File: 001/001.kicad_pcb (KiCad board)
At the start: 2 copper layers, 47.6 x 49.1 mm, 8 parts, among them U1 MF-Jalisco, U2 Firma, U3 PinBase

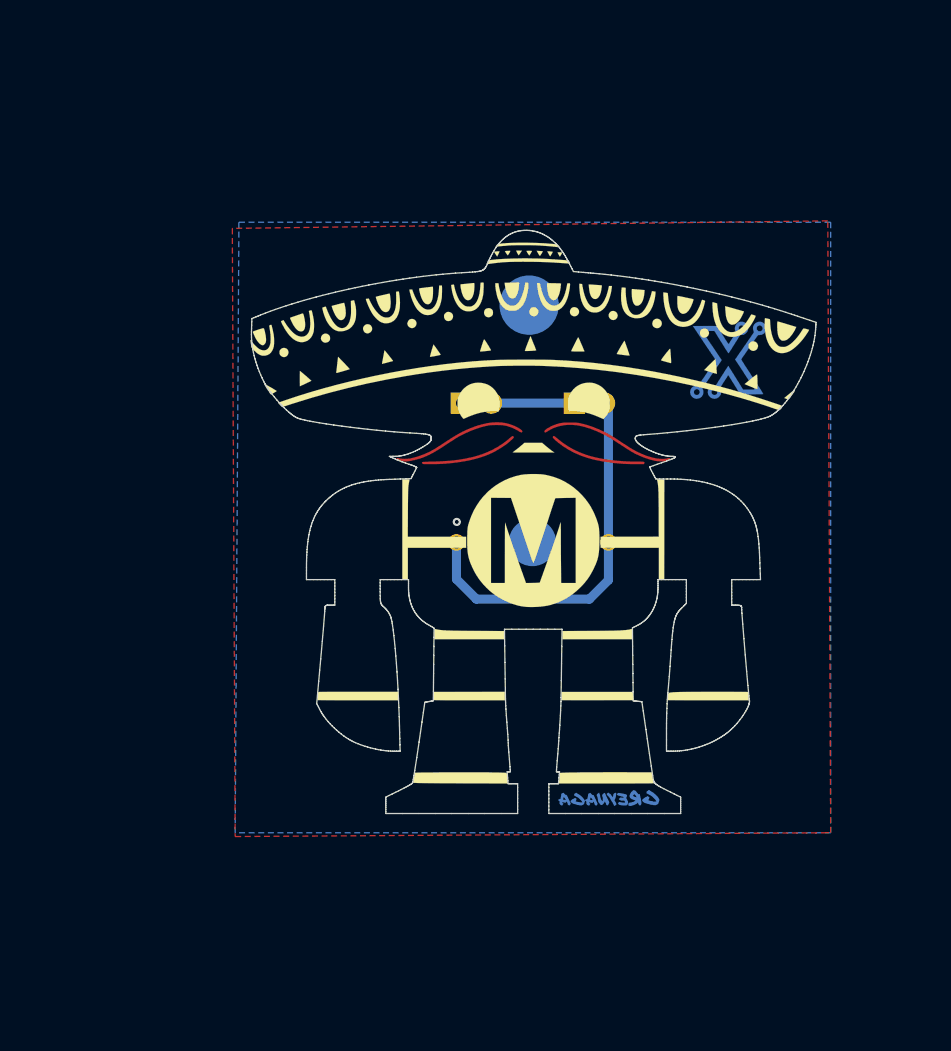
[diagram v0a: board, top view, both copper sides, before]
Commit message: Changes
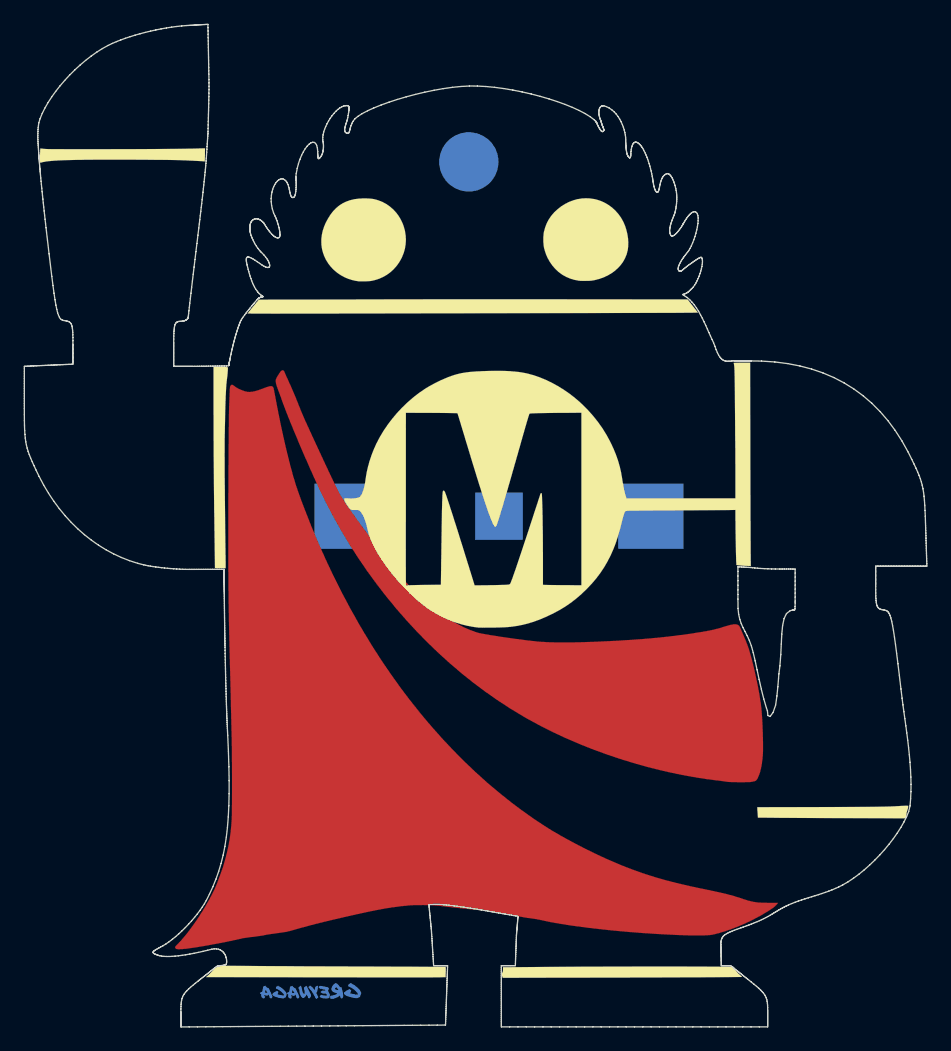
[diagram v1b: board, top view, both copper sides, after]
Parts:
- removed the Ref** at (153.7, 87.0)
- removed the Ref** at (123.1, 87.9)
- removed U1: MF-Jalisco, MF-Jalisco:MF-Jalisco_50mm
- added Ref**: Val**, MF-ROME:Rome_100mm_01, F.Cu at (134.0, 102.9)
- BT1: footprint MF-Jalisco:CR1220-Jalisco -> MF-ROME:S8211R
- D1, D2: footprint MF-Jalisco:LED_D5.0mm_FlatTop -> MF-ROME:LED_D5.0mm_FlatTop
- U2: footprint MF-Jalisco:firma_Cu_Mask -> MF-ROME:firma_Cu_Mask
- U3: footprint MF-Jalisco:PinBase -> MF-ROME:PinBase
- moved U2 29.9 mm to (118.7, 139.7)
- moved D1 16.8 mm to (121.8, 76.5)
- moved D2 13.7 mm to (140.6, 76.5)
- moved U3 13.1 mm to (132.1, 69.8)
- moved BT1 3.58 mm to (134.6, 99.7), turned to 180 degrees
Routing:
- net +3V3: track 32.3 -> 0.00 mm
- net Net-(D1-Pad2): track 6.98 -> 0.00 mm
- net GND: vias 1 -> 0
- removed copper zone on B.Cu, net GND
- removed copper zone on F.Cu, net GND
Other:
- board size 47.6 x 49.1 mm -> 76 x 84.5 mm
- board text removed: "Developed by"
